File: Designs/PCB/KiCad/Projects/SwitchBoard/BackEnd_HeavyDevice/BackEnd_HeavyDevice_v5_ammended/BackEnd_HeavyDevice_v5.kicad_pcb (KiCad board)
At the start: 2 copper layers, 21 parts, among them J2 Screw_Terminal_01x02, J3 Conn_01x06_Female, J5 Screw_Terminal_01x02, M1 MountingHole_2.1mm, M2 MountingHole_2.1mm, Q1 BT136-500, U2 ACS712-20, U3 4N35, U4 AP2112K-3.3, U5 MOC3021

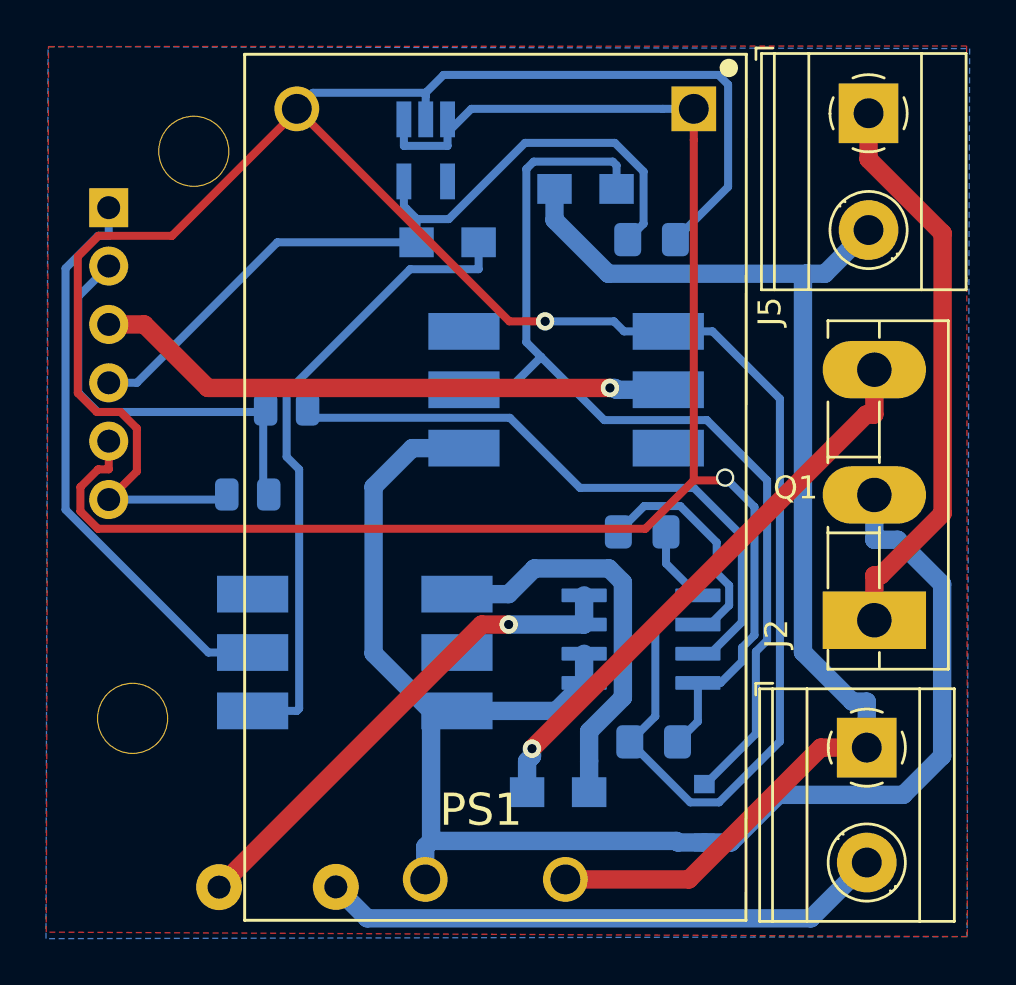
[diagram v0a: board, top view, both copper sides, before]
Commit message: update_29-05-2022
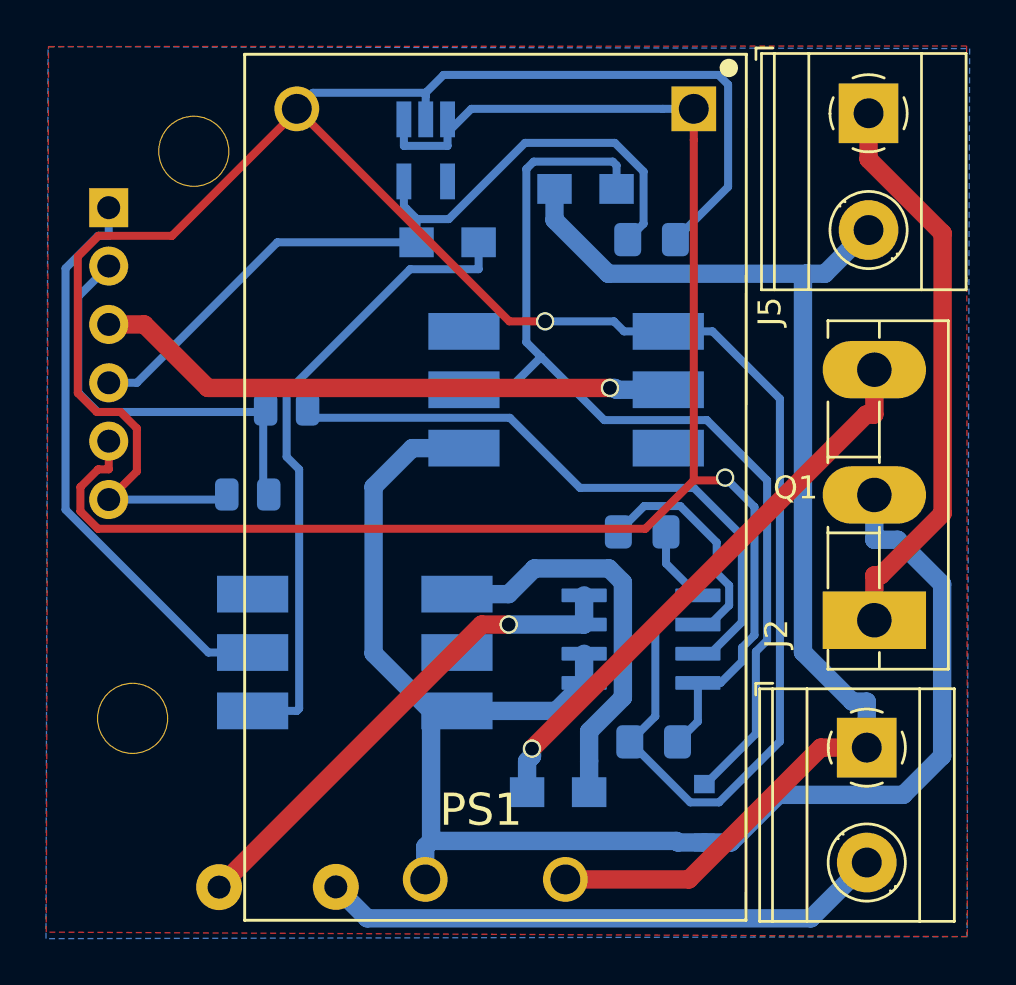
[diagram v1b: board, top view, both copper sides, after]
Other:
- net class AC removed
- net class Default removed
